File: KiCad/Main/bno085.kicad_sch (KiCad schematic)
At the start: 11 parts, among them J7 RJ45, J9 RJ45

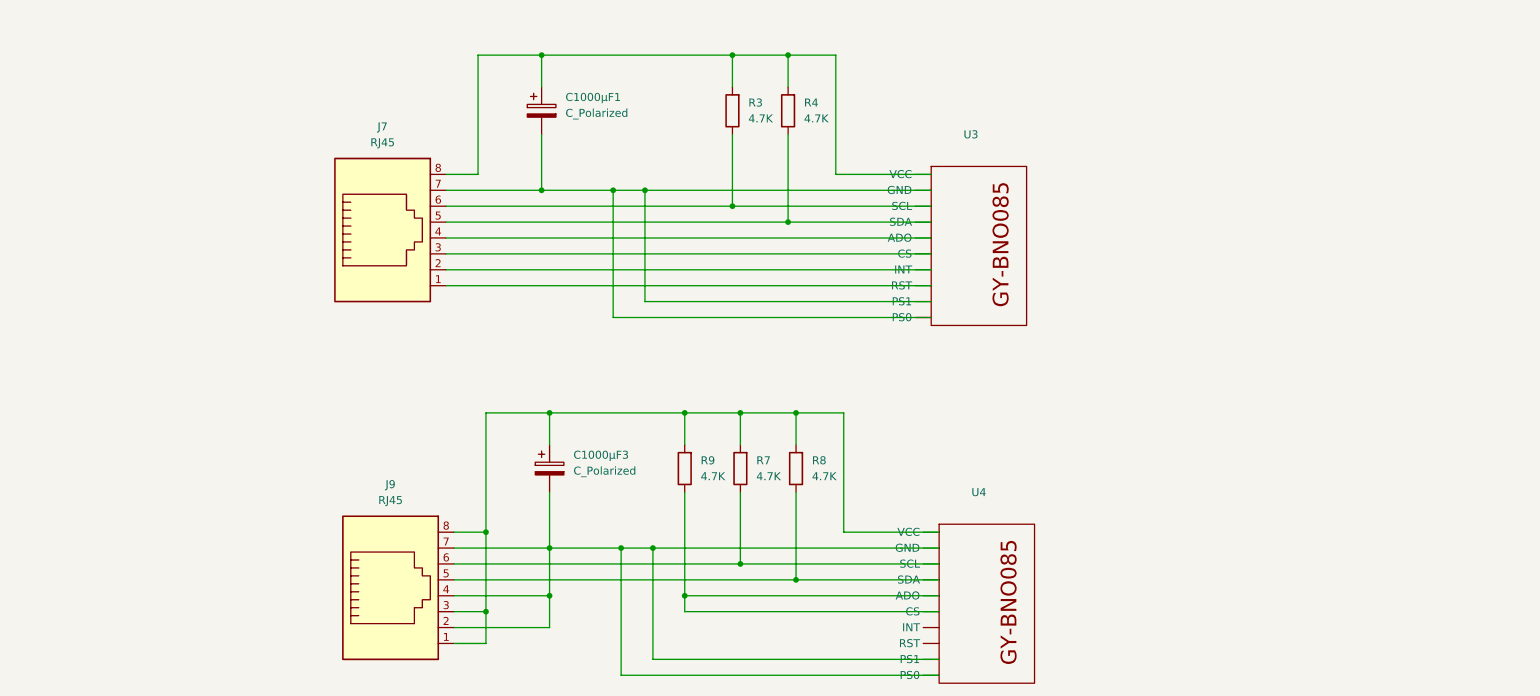
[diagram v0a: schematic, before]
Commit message: bno085 et moteurs OK
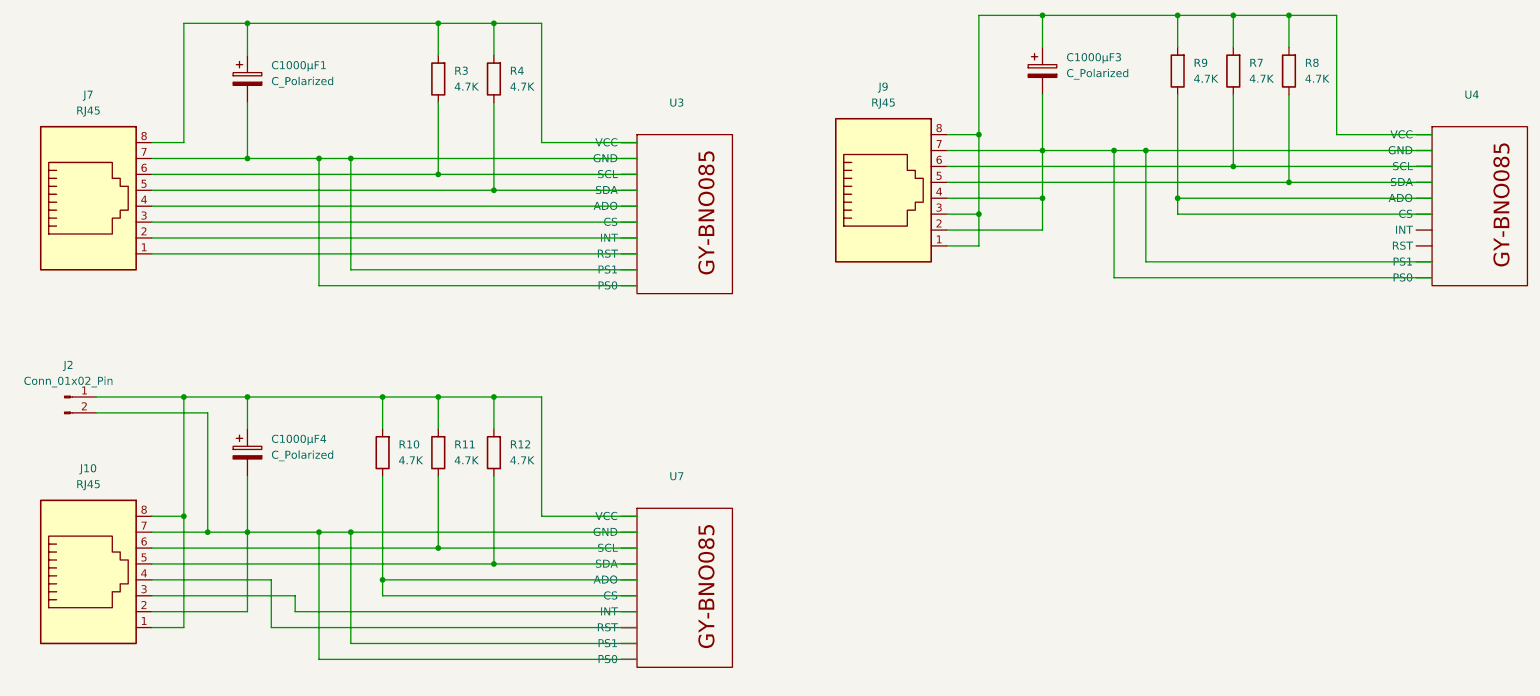
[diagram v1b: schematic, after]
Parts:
- added C1000µF4: C_Polarized, Capacitor_THT:CP_Radial_D17.0mm_P7.50mm, symbol Device:C_Polarized
- added J10: RJ45, Connector_RJ:RJ45_Amphenol_54602-x08_Horizontal, symbol Connector:RJ45
- added J2: Conn_01x02_Pin, symbol Connector:Conn_01x02_Pin
- added R10, R11, R12: 4.7K, symbol Device:R
- added U7: (no value), symbol gy-bno08x:gy-bno08x
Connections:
- net at U4. (PS0): now also R9.1
- new net: J10.6, R11.1, U7. (PS0)
- new net: C1000µF4.1, J10.1, J10.8, J2.1 (Pin_1), R10.2, R11.2, R12.2, U7. (PS0)
- new net: C1000µF4.2, J10.2, J10.7, J2.2 (Pin_2), U7. (PS0)
- new net: J10.3, U7. (PS0)
- new net: J10.4, U7. (PS0)
- new net: J10.5, R12.1, U7. (PS0)
- new net: R10.1, U7. (PS0)
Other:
- moved on the sheet: C1000µF1, C1000µF3, J7, J9, R3, R4, R7, R8, R9, U3, U4
